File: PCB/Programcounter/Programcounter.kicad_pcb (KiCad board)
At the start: 2 copper layers, 102 x 102 mm, 86 parts, among them U1 74LS541, U10 74LS157, U11 74LS157, U12 74LS157, U13 74LS157, U14 74LS157, U15 74LS157, U2 74LS541, U3 74LS541, U4 74LS163, U5 74LS163, U6 74LS163, U7 74LS163, U8 74LS163, U9 74LS163

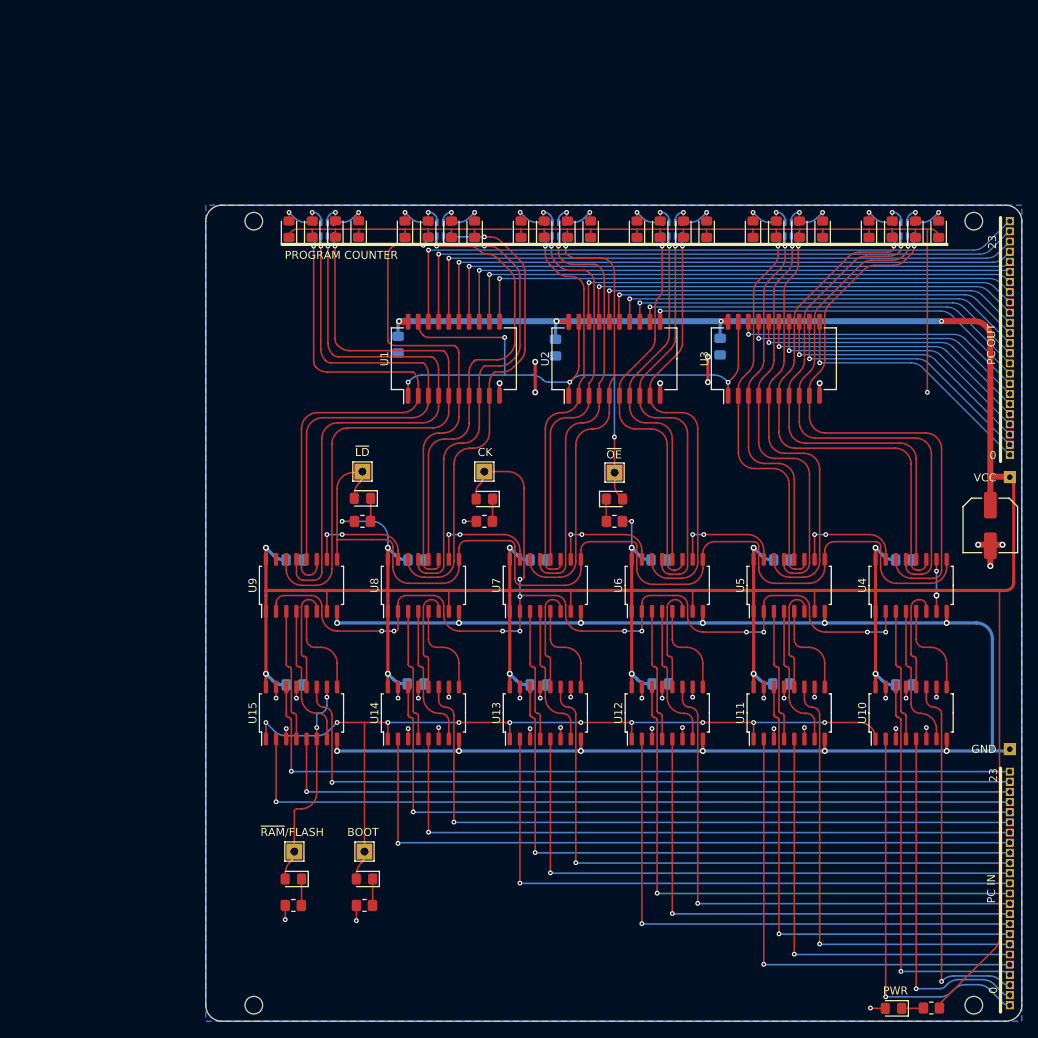
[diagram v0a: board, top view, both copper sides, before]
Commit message: WIP
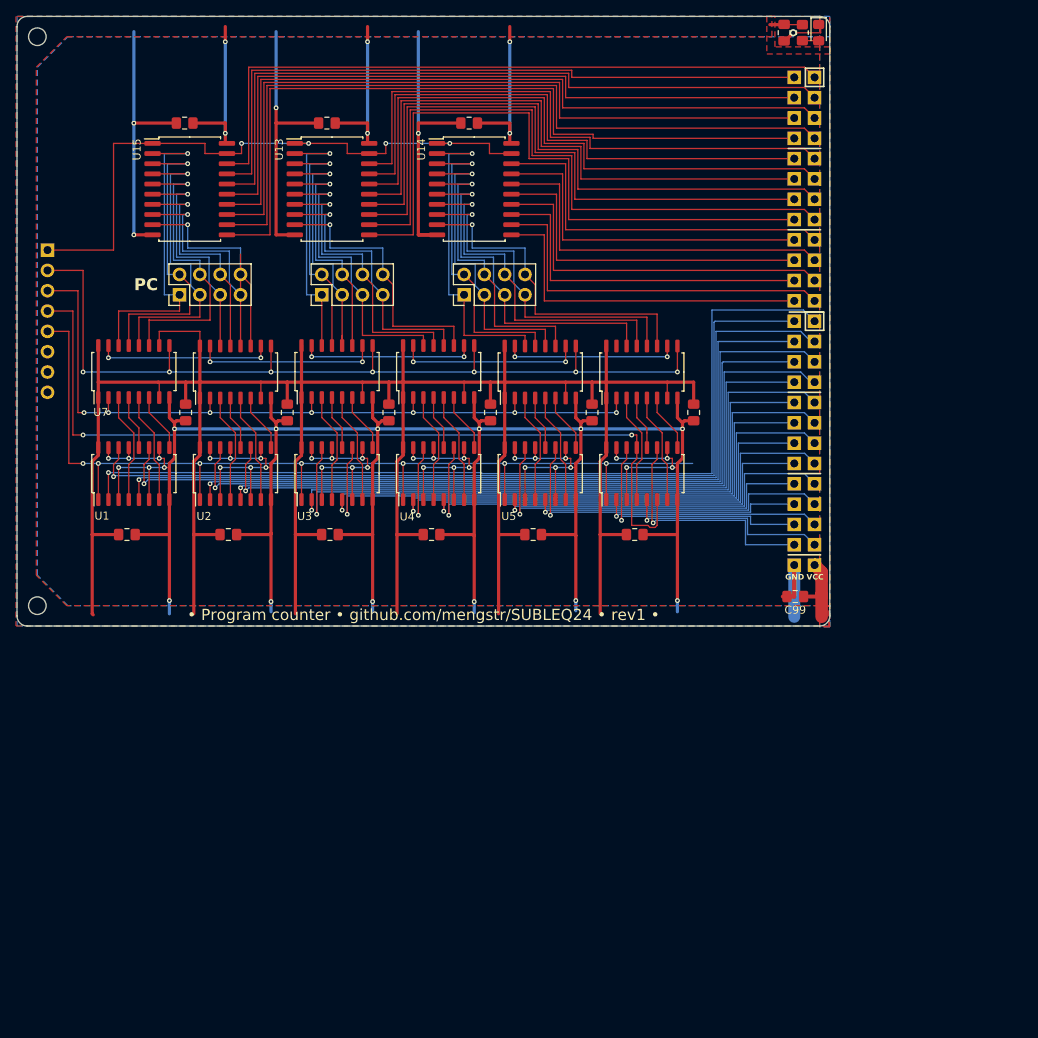
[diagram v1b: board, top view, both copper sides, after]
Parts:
- removed C16, C17, C18: C, Capacitor_SMD:C_0805_2012Metric_Pad1.18x1.45mm_HandSolder
- removed D1, D10, D11, D12, D13, D14, D15, D16, D17, D18, D19, D2, D20, D21, D22, D23, D24, D25, D26, D27, D28, D29, D3, D30, D4, D5, D6, D7, D8, D9: LED, LED_SMD:LED_0805_2012Metric_Pad1.15x1.40mm_HandSolder
- removed H3, H4: MountingHole, matseng:MountingHole_M2
- removed JBOTRIGHT1, JTOPRIGHT1: Conn_01x24, matseng:PinHeader_1x24_P1.27mm_NoSilk
- removed R1, R2, R3, R4, R5, R6: R, Resistor_SMD:R_0805_2012Metric_Pad1.20x1.40mm_HandSolder
- removed RN1, RN2, RN3, RN4, RN5, RN6: R_Pack04, Resistor_SMD:R_Array_Concave_4x0603
- removed TP1, TP4, TP5, TP7, TP8: TestPoint, TestPoint:TestPoint_THTPad_2.0x2.0mm_Drill1.0mm
- removed TP2, TP3: TestPoint, TestPoint:TestPoint_THTPad_1.5x1.5mm_Drill0.7mm
- added BUS1: Conn_02x25_Odd_Even, Connector_PinHeader_2.54mm:PinHeader_2x25_P2.54mm_Vertical, B.Cu at (125.1, 33.0)
- added C2: C, Capacitor_SMD:C_0805_2012Metric_Pad1.18x1.45mm_HandSolder, F.Cu at (102.6, 90.2)
- added C8: C, Capacitor_SMD:C_0805_2012Metric_Pad1.18x1.45mm_HandSolder, F.Cu at (97.3, 74.9)
- added C98: C, Capacitor_SMD:C_0805_2012Metric_Pad1.18x1.45mm_HandSolder, F.Cu at (121.3, 27.4)
- added C99: C, Capacitor_SMD:C_0805_2012Metric_Pad1.18x1.45mm_HandSolder, F.Cu at (122.7, 97.9)
- added D99: LED, LED_SMD:LED_0805_2012Metric_Pad1.15x1.40mm_HandSolder, F.Cu at (125.6, 27.4)
- added J1a1: Conn_02x04_Odd_Even, Connector_PinHeader_2.54mm:PinHeader_2x04_P2.54mm_Vertical, F.Cu at (45.7, 60.2)
- added J1b1: Conn_02x04_Odd_Even, Connector_PinHeader_2.54mm:PinHeader_2x04_P2.54mm_Vertical, F.Cu at (63.5, 60.2)
- added J1c1: Conn_02x04_Odd_Even, Connector_PinHeader_2.54mm:PinHeader_2x04_P2.54mm_Vertical, F.Cu at (81.3, 60.2)
- added J3: Conn_01x08_Pin, Connector_PinHeader_2.54mm:PinHeader_1x08_P2.54mm_Vertical, B.Cu at (29.2, 54.6)
- added R99: R, Resistor_SMD:R_0805_2012Metric_Pad1.20x1.40mm_HandSolder, F.Cu at (123.6, 27.4)
- C1: footprint Capacitor_SMD:C_Elec_6.3x5.8 -> Capacitor_SMD:C_0805_2012Metric_Pad1.18x1.45mm_HandSolder
- C10, C11, C12, C13, C14, C15, C3, C4, C5, C6, C7, C9: moved to F.Cu
- U1, U2, U3: value 74LS541 -> 74LS157; footprint Package_SO:SOIC-20W_7.5x15.4mm_P1.27mm -> Package_SO:SOIC-16_4.55x10.3mm_P1.27mm
- U10, U11, U12: value 74LS157 -> 74LS163
- U13, U14, U15: value 74LS157 -> 74LS541; footprint Package_SO:SOIC-16_4.55x10.3mm_P1.27mm -> Package_SO:SOIC-20W_7.5x12.8mm_P1.27mm
- U4, U5, U6: value 74LS163 -> 74LS157
- moved H1 168.4 mm to (27.9, 27.9)
- moved C6 98.9 mm to (39.1, 90.2)
- moved C7 81.8 mm to (46.5, 74.9), turned to -90 degrees
- moved C15 80.6 mm to (46.4, 38.7), turned to 180 degrees
- moved C13 75.0 mm to (64.1, 38.7), turned to 180 degrees
- moved U10 72.9 mm to (78.1, 69.8)
- moved U13 70.7 mm to (64.8, 47.0), turned to 0 degrees
- moved C4 67.0 mm to (71.9, 74.9), turned to -90 degrees
- moved U15 67.0 mm to (47.0, 47.0), turned to 0 degrees
- moved U14 65.8 mm to (82.5, 47.0), turned to 0 degrees
- moved C1 64.1 mm to (84.6, 74.9)
- moved U4 60.7 mm to (78.1, 82.5)
- moved U7 58.0 mm to (40.0, 69.8)
- moved H2 56.8 mm to (27.9, 99.1)
- moved U3 56.5 mm to (65.4, 82.5)
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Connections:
- U1 pad 1: /~{OE} -> /SEL
- U1 pad 11: /BUS16 -> /D3
- U1 pad 12: /BUS17 -> /New1
- U1 pad 13: /BUS18 -> GNDD
- U1 pad 14: /BUS19 -> /D1
- U1 pad 15: /BUS20 -> GNDD
- U1 pad 16: /BUS21 -> VCC
- U1 pad 2: /PC23 -> /D0
- U1 pad 3: /PC22 -> GNDD
- U1 pad 4: /PC21 -> /New0
- U1 pad 5: /PC20 -> /D2
- U1 pad 6: /PC19 -> GNDD
- U1 pad 7: /PC18 -> /New2
- U1 pad 8: /PC17 -> GNDD
- U1 pad 9: /PC16 -> /New3
- U10 pad 1: /SEL -> VCC
- U10 pad 10: GNDD -> Net-(U10-CET)
- U10 pad 11: /IN2 -> /PC15
- U10 pad 12: /NEWCNT3 -> /PC14
- U10 pad 13: GNDD -> /PC13
- U10 pad 14: /IN3 -> /PC12
- U10 pad 15: GNDD -> Net-(U10-TC)
- U10 pad 2: /IN0 -> /CP
- U10 pad 3: GNDD -> /New12
- U10 pad 4: /NEWCNT0 -> /New13
- U10 pad 5: /IN1 -> /New14
- U10 pad 6: GNDD -> /New15
- U10 pad 7: /NEWCNT1 -> VCC
- U10 pad 9: /NEWCNT2 -> /~{PE}
- U11 pad 1: /SEL -> VCC
- U11 pad 10: GNDD -> Net-(U10-TC)
- U11 pad 11: /IN6 -> /PC19
- U11 pad 12: /NEWCNT7 -> /PC18
- U11 pad 13: GNDD -> /PC17
- U11 pad 14: /IN7 -> /PC16
- U11 pad 15: GNDD -> Net-(U11-TC)
- U11 pad 2: /IN4 -> /CP
- U11 pad 3: GNDD -> /New16
- U11 pad 4: /NEWCNT4 -> /New17
- U11 pad 5: /IN5 -> /New18
- U11 pad 6: GNDD -> /New19
- U11 pad 7: /NEWCNT5 -> VCC
- U11 pad 9: /NEWCNT6 -> /~{PE}
- U12 pad 1: /SEL -> VCC
- U12 pad 10: GNDD -> Net-(U11-TC)
- U12 pad 11: /IN10 -> /PC23
- U12 pad 12: /NEWCNT11 -> /PC22
- U12 pad 13: GNDD -> /PC21
- U12 pad 14: /IN11 -> /PC20
- U12 pad 15: GNDD -> unconnected-(U12-TC-Pad15)
- U12 pad 2: /IN8 -> /CP
- U12 pad 3: GNDD -> /New20
- U12 pad 4: /NEWCNT8 -> /New21
- U12 pad 5: /IN9 -> /New22
- U12 pad 6: GNDD -> /New23
- U12 pad 7: /NEWCNT9 -> VCC
- U12 pad 9: /NEWCNT10 -> /~{PE}
- U13 pad 1: /SEL -> /~{OE}
- U13 pad 11: /IN14 -> /A15
- U13 pad 12: /NEWCNT15 -> /A14
- U13 pad 13: GNDD -> /A13
- U13 pad 14: /IN15 -> /A12
- U13 pad 15: GNDD -> /A11
- U13 pad 16: VCC -> /A10
- U13 pad 2: /IN12 -> /PC8
- U13 pad 3: GNDD -> /PC9
- U13 pad 4: /NEWCNT12 -> /PC10
- U13 pad 5: /IN13 -> /PC11
- U13 pad 6: GNDD -> /PC12
- U13 pad 7: /NEWCNT13 -> /PC13
- U13 pad 8: GNDD -> /PC14
- U13 pad 9: /NEWCNT14 -> /PC15
- U14 pad 1: /SEL -> /~{OE}
- U14 pad 11: /IN18 -> /A23
- U14 pad 12: /NEWCNT19 -> /A22
- U14 pad 13: GNDD -> /A21
- U14 pad 14: /IN19 -> /A20
- U14 pad 15: GNDD -> /A19
- U14 pad 16: VCC -> /A18
- U14 pad 2: /IN16 -> /PC16
- U14 pad 3: GNDD -> /PC17
- U14 pad 4: /NEWCNT16 -> /PC18
- U14 pad 5: /IN17 -> /PC19
- U14 pad 6: GNDD -> /PC20
- U14 pad 7: /NEWCNT17 -> /PC21
- U14 pad 8: GNDD -> /PC22
- U14 pad 9: /NEWCNT18 -> /PC23
- U15 pad 1: /SEL -> /~{OE}
- U15 pad 10: /BOOTADDR -> GNDD
- U15 pad 11: /IN22 -> /A7
- U15 pad 12: /NEWCNT23 -> /A6
- U15 pad 13: GNDD -> /A5
- U15 pad 14: /IN23 -> /A4
- U15 pad 15: GNDD -> /A3
- U15 pad 16: VCC -> /A2
- U15 pad 2: /IN20 -> /PC0
- U15 pad 3: GNDD -> /PC1
- U15 pad 4: /NEWCNT20 -> /PC2
- U15 pad 5: /IN21 -> /PC3
- U15 pad 6: /BOOTADDR -> /PC4
- U15 pad 7: /NEWCNT21 -> /PC5
- U15 pad 8: GNDD -> /PC6
- U15 pad 9: /NEWCNT22 -> /PC7
- U2 pad 1: /~{OE} -> /SEL
- U2 pad 11: /BUS8 -> /D7
- U2 pad 12: /BUS9 -> /New5
- U2 pad 13: /BUS10 -> GNDD
- U2 pad 14: /BUS11 -> /D5
- U2 pad 15: /BUS12 -> GNDD
- U2 pad 16: /BUS13 -> VCC
- U2 pad 2: /PC15 -> /D4
- U2 pad 3: /PC14 -> GNDD
- U2 pad 4: /PC13 -> /New4
- U2 pad 5: /PC12 -> /D6
- U2 pad 6: /PC11 -> GNDD
- U2 pad 7: /PC10 -> /New6
- U2 pad 8: /PC9 -> GNDD
- U2 pad 9: /PC8 -> /New7
- U3 pad 1: /~{OE} -> /SEL
- U3 pad 11: /BUS0 -> /D11
- U3 pad 12: /BUS1 -> /New9
- U3 pad 13: /BUS2 -> GNDD
- U3 pad 14: /BUS3 -> /D9
- U3 pad 15: /BUS4 -> GNDD
- U3 pad 16: /BUS5 -> VCC
- U3 pad 2: /PC7 -> /D8
- U3 pad 3: /PC6 -> GNDD
- U3 pad 4: /PC5 -> /New8
- U3 pad 5: /PC4 -> /D10
- U3 pad 6: /PC3 -> GNDD
- U3 pad 7: /PC2 -> /New10
- U3 pad 8: /PC1 -> GNDD
- U3 pad 9: /PC0 -> /New11
- U4 pad 1: VCC -> /SEL
- U4 pad 10: VCC -> GNDD
- U4 pad 11: /PC3 -> /D15
- U4 pad 12: /PC2 -> /New13
- U4 pad 13: /PC1 -> GNDD
- U4 pad 14: /PC0 -> /D13
- U4 pad 15: Net-(U4-TC) -> GNDD
- U4 pad 2: /CP -> /D12
- U4 pad 3: /NEWCNT0 -> GNDD
- U4 pad 4: /NEWCNT1 -> /New12
- U4 pad 5: /NEWCNT2 -> /D14
- U4 pad 6: /NEWCNT3 -> GNDD
- U4 pad 7: VCC -> /New14
- U4 pad 9: /~{PE} -> /New15
- U5 pad 1: VCC -> /SEL
- U5 pad 10: Net-(U4-TC) -> GNDD
- U5 pad 11: /PC7 -> /D19
- U5 pad 12: /PC6 -> /New17
- U5 pad 13: /PC5 -> GNDD
- U5 pad 14: /PC4 -> /D17
- U5 pad 15: Net-(U5-TC) -> GNDD
- U5 pad 2: /CP -> /D16
- U5 pad 3: /NEWCNT4 -> GNDD
- U5 pad 4: /NEWCNT5 -> /New16
- U5 pad 5: /NEWCNT6 -> /D18
- U5 pad 6: /NEWCNT7 -> GNDD
- U5 pad 7: VCC -> /New18
- U5 pad 9: /~{PE} -> /New19
- U6 pad 1: VCC -> /SEL
- U6 pad 10: Net-(U5-TC) -> GNDD
- U6 pad 11: /PC11 -> /D23
- U6 pad 12: /PC10 -> /New21
- U6 pad 13: /PC9 -> /BootAddr
- U6 pad 14: /PC8 -> /D21
- U6 pad 15: Net-(U6-TC) -> GNDD
- U6 pad 2: /CP -> /D20
- U6 pad 3: /NEWCNT8 -> GNDD
- U6 pad 4: /NEWCNT9 -> /New20
- U6 pad 5: /NEWCNT10 -> /D22
- U6 pad 6: /NEWCNT11 -> /BootAddr
- U6 pad 7: VCC -> /New22
- U6 pad 9: /~{PE} -> /New23
- U7 pad 10: Net-(U6-TC) -> VCC
- U7 pad 11: /PC15 -> /PC3
- U7 pad 12: /PC14 -> /PC2
- U7 pad 13: /PC13 -> /PC1
- U7 pad 14: /PC12 -> /PC0
- U7 pad 3: /NEWCNT12 -> /New0
- U7 pad 4: /NEWCNT13 -> /New1
- U7 pad 5: /NEWCNT14 -> /New2
- U7 pad 6: /NEWCNT15 -> /New3
- U8 pad 11: /PC19 -> /PC7
- U8 pad 12: /PC18 -> /PC6
- U8 pad 13: /PC17 -> /PC5
- U8 pad 14: /PC16 -> /PC4
- U8 pad 3: /NEWCNT16 -> /New4
- U8 pad 4: /NEWCNT17 -> /New5
- U8 pad 5: /NEWCNT18 -> /New6
- U8 pad 6: /NEWCNT19 -> /New7
- U9 pad 11: /PC23 -> /PC11
- U9 pad 12: /PC22 -> /PC10
- U9 pad 13: /PC21 -> /PC9
- U9 pad 14: /PC20 -> /PC8
- U9 pad 15: unconnected-(U9-TC-Pad15) -> Net-(U10-CET)
- U9 pad 3: /NEWCNT20 -> /New8
- U9 pad 4: /NEWCNT21 -> /New9
- U9 pad 5: /NEWCNT22 -> /New10
- U9 pad 6: /NEWCNT23 -> /New11
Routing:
- net GNDD: track 387.3 -> 536.9 mm, vias 55 -> 51
- net /D0: track 0.00 -> 112.7 mm, vias 0 -> 1
- net /D1: track 0.00 -> 108.3 mm, vias 0 -> 1
- net /BootAddr: track 0.00 -> 107.3 mm, vias 0 -> 2
- net /D2: track 0.00 -> 105.9 mm, vias 0 -> 1
- net /D3: track 0.00 -> 103.5 mm, vias 0 -> 1
- net /IN23: track 100.7 -> 0.00 mm, vias 1 -> 0
- net /IN20: track 99.6 -> 0.00 mm, vias 1 -> 0
- net /IN22: track 97.7 -> 0.00 mm, vias 1 -> 0
- net /A6: track 0.00 -> 96.7 mm
- net /A7: track 0.00 -> 95.4 mm
- net /IN21: track 94.5 -> 0.00 mm, vias 1 -> 0
- net /D4: track 0.00 -> 94.4 mm, vias 0 -> 1
- net /A4: track 0.00 -> 93.2 mm
- net /D5: track 0.00 -> 93.1 mm, vias 0 -> 1
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- added copper zone on F.Cu, net VCC
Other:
- board size 102 x 102 mm -> 101.6 x 76.2 mm
- board text added: "PC"
- board text added: "• Program counter • github.com/mengstr/SUBLEQ24 • rev1 •"
- board text removed: "0"
- board text removed: "23"
- board text removed: "BOOT"
- board text removed: "CK"
- board text removed: "DISCRETE 24 BIT SUBLEQ PROGRAM COUNTER GITHUB.COM/MENGSTR/SUBLEQ24 30 OCTOBER 2023"
- board text removed: "PC IN"
- board text removed: "PC OUT"
- board text removed: "PROGRAM COUNTER"
- board text removed: "PWR"
- board text removed: "~{LD}"
- board text removed: "~{OE}"
- board text removed: "~{RAM}/FLASH"
